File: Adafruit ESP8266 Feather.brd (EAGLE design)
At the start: 50.8 x 22.9 mm, 40 parts, among them IC1 CP2104, Q1 mmbt2222, Q2 mmbt2222, SW2 KMR2, U2 SPX3819, U3 MCP73831T-2ACI/OT, X1 JSTPH, X2 ESP-12, X4 20329

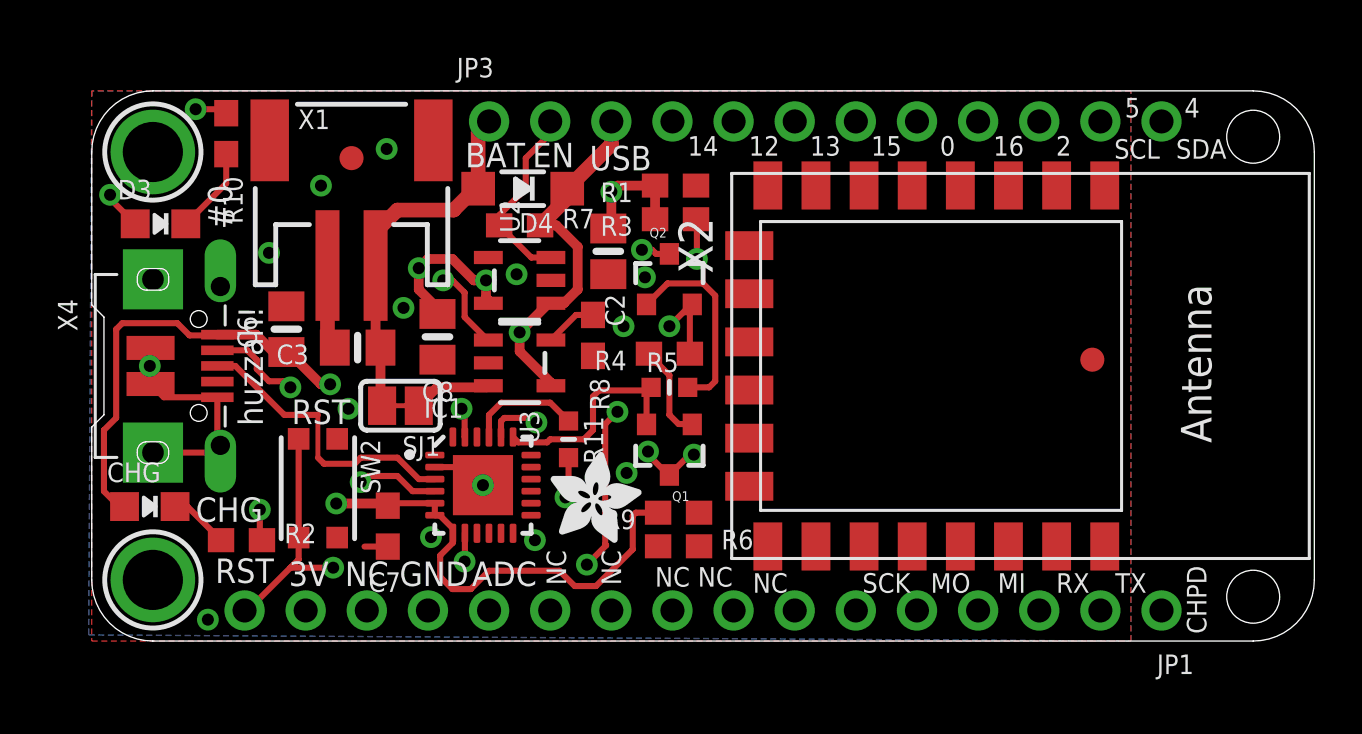
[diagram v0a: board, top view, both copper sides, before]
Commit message: Feather .Brd: minor adjustments
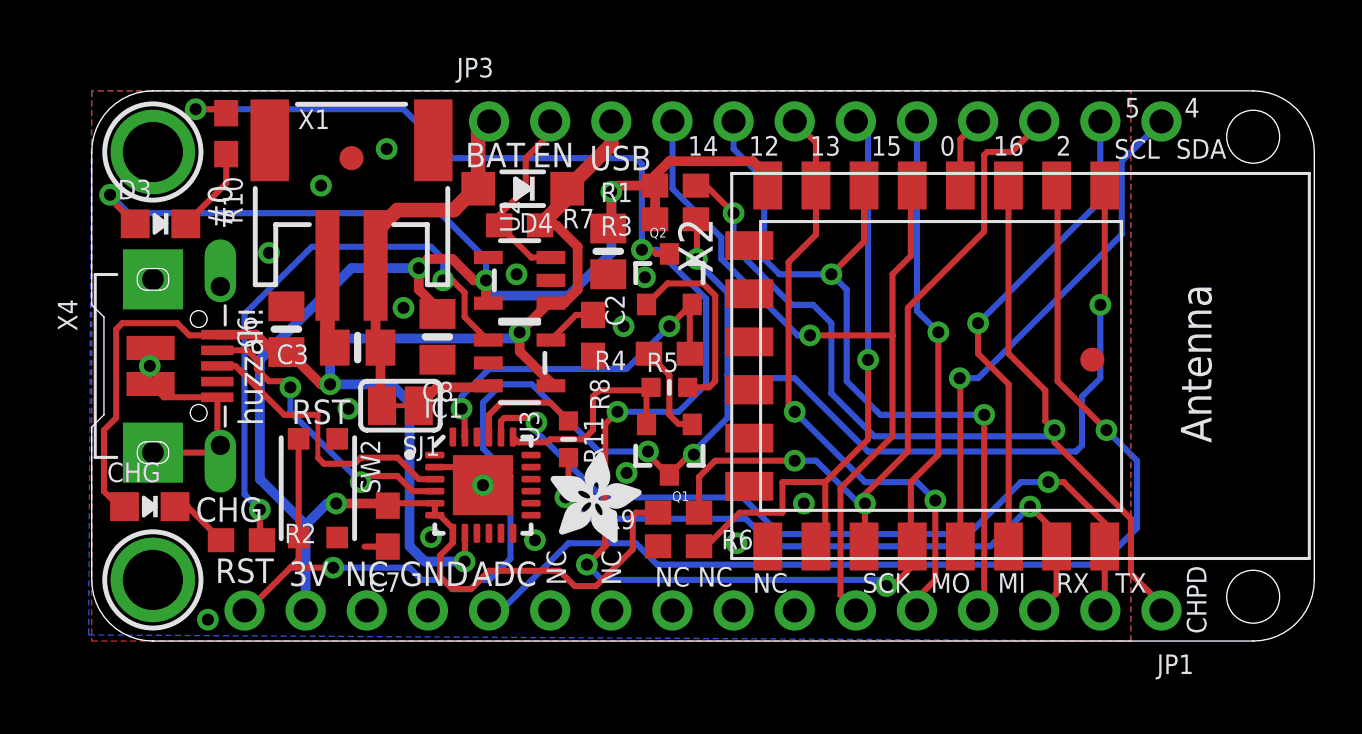
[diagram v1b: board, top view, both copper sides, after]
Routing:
- net GPIO0: track 9.46 -> 77.7 mm, vias 4 -> 6
- net RESET: track 14.3 -> 74.4 mm, vias 4 -> 5
- net 3.3V: track 32.9 -> 86.4 mm
- net ADC: track 0.00 -> 44.7 mm, vias 0 -> 1
- net CH_PD: track 0.71 -> 42.4 mm, vias 0 -> 2
- net GPIO14/SCK: track 0.00 -> 34.1 mm, vias 0 -> 1
- net GPIO12/MISO: track 0.00 -> 32.8 mm, vias 0 -> 2
- net TXD: track 2.26 -> 33.3 mm, vias 1 -> 2
- net GPIO2: track 0.13 -> 30.7 mm, vias 0 -> 2
- net RXD: track 1.70 -> 27.6 mm, vias 1 -> 2
- net GPIO15: track 0.29 -> 25.9 mm, vias 0 -> 1
- net GPIO13/MOSI: track 0.00 -> 25.3 mm, vias 0 -> 2
- net VBUS: track 34.5 -> 56.3 mm
- net GPIO4/SDA: track 0.00 -> 21.6 mm, vias 0 -> 1
- net GPIO5/SCL: track 0.00 -> 20.3 mm, vias 0 -> 1
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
